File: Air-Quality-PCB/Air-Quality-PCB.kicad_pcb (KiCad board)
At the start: 2 copper layers, 98.4 x 93.7 mm, 48 parts, among them J1 Conn_01x03_Female, J10 Conn_01x02_Female, J11 Conn_01x10_Female, J12 Conn_01x02_Female, J13 Conn_01x10_Female, J14 Conn_01x03_Female, J15 Conn_01x03_Female, J16 Conn_01x04_Female, J17 Conn_01x04_Female, J18 Conn_01x05_Female, J19 Conn_01x05_Female, J2 Conn_01x10_Female, J20 Conn_01x04_Female, J21 Conn_01x03_Female, J3 Conn_01x08_Female, J4 Conn_01x10_Female, J5 Conn_01x03_Female, J6 Conn_01x03_Female, J7 Conn_01x07_Female, J8 Conn_01x07_Female, J9 Conn_01x04_Female, Q1 AO3401A, Q2 AO3401A, Q3 2N7002E, Q4 2N7002E, Q5 AO3401A, Q6 AO3401A, Q7 AO3401A

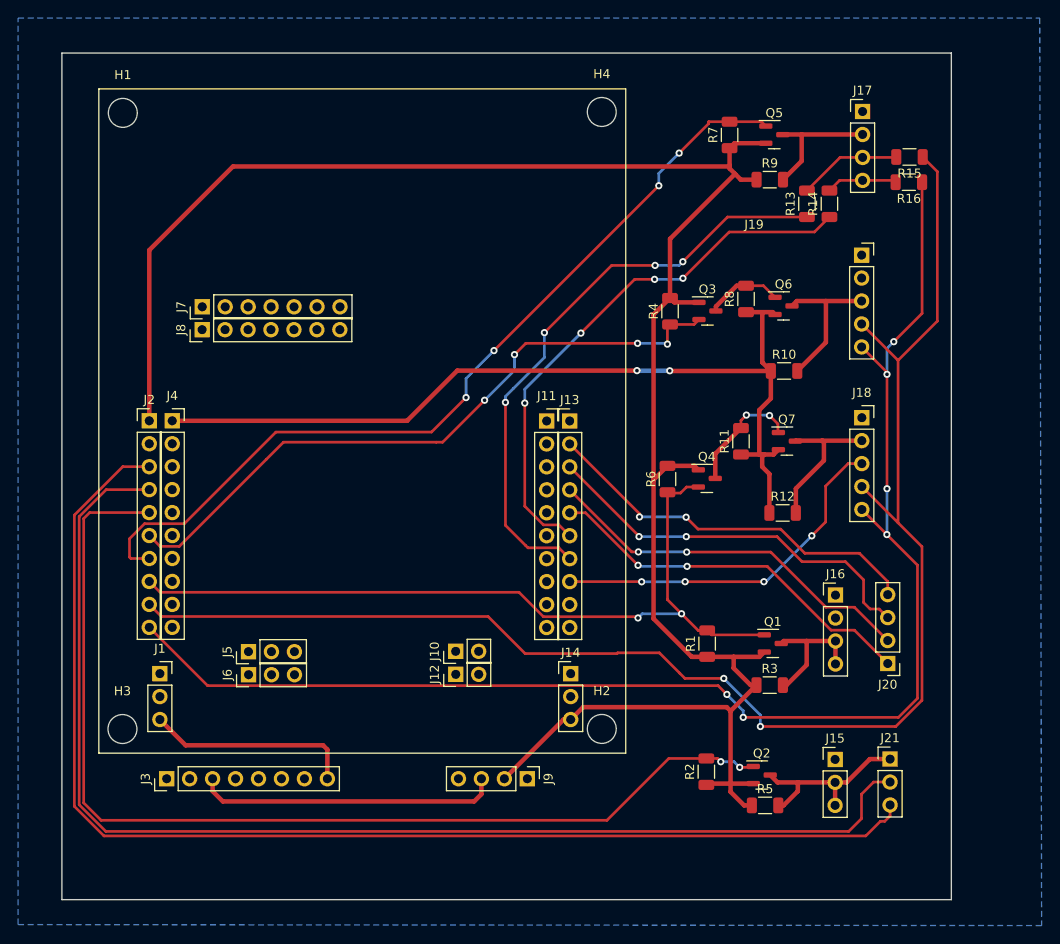
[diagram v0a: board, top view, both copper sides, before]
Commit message: Add files via upload
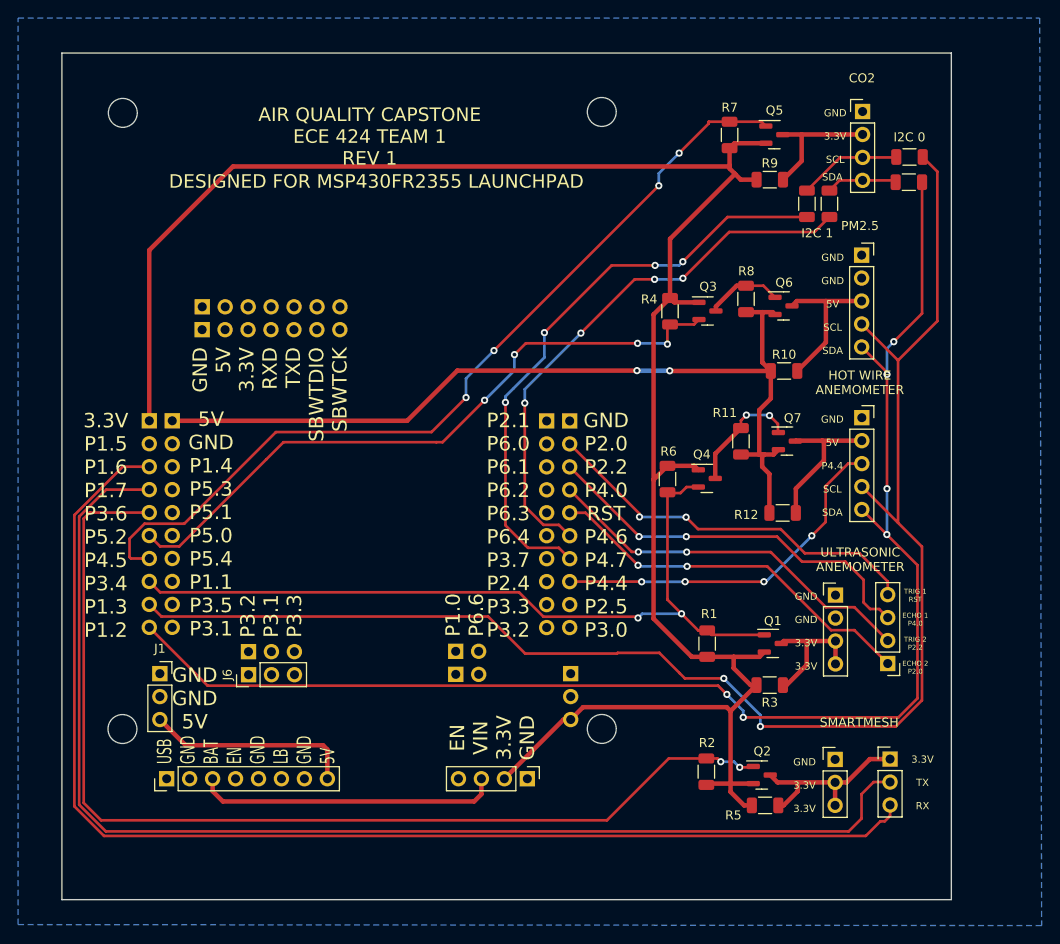
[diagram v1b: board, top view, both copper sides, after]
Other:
- board text added: "3.3V P1.5 P1.6 P1.7 P3.6 P5.2 P4.5 P3.4 P1.3 P1.2"
- board text added: "3.3V TX RX"
- board text added: "5V GND P1.4 P5.3 P5.1 P5.0 P5.4 P1.1 P3.5 P3.1"
- board text added: "AIR QUALITY CAPSTONE ECE 424 TEAM 1 REV 1"
- board text added: "CO2"
- board text added: "DESIGNED FOR MSP430FR2355 LAUNCHPAD"
- board text added: "EN VIN 3.3V GND"
- board text added: "GND 3.3V 3.3V"
- board text added: "GND 3.3V SCL"
- board text added: "GND 5V 3.3V RXD TXD SBWTDIO SBWTCK"
- board text added: "GND 5V P4.4 SCL SDA"
- board text added: "GND GND 3.3V 3.3V"
- board text added: "GND GND 5V"
- board text added: "GND GND 5V SCL SDA"
- board text added: "GND P2.0 P2.2 P4.0 RST P4.6 P4.7 P4.4 P2.5 P3.0"
- board text added: "HOT WIRE ANEMOMETER"
- board text added: "I2C 0"
- board text added: "I2C 1"
- board text added: "P1.0 P6.6"
- board text added: "P2.1 P6.0 P6.1 P6.2 P6.3 P6.4 P3.7 P2.4 P3.3 P3.2"
- board text added: "P3.2 P3.1 P3.3"
- board text added: "PM2.5"
- board text added: "SDA"
- board text added: "SMARTMESH"
- board text added: "TRIG 1 RST ECHO 1 P4.0 TRIG 2 P2.2 ECHO 2 P2.0"
- board text added: "ULTRASONIC ANEMOMETER"
- board text added: "USB GND BAT EN GND LB GND 5V"
